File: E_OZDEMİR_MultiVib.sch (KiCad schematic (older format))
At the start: 11 parts, among them U1 MJB41C, U2 MJB41C

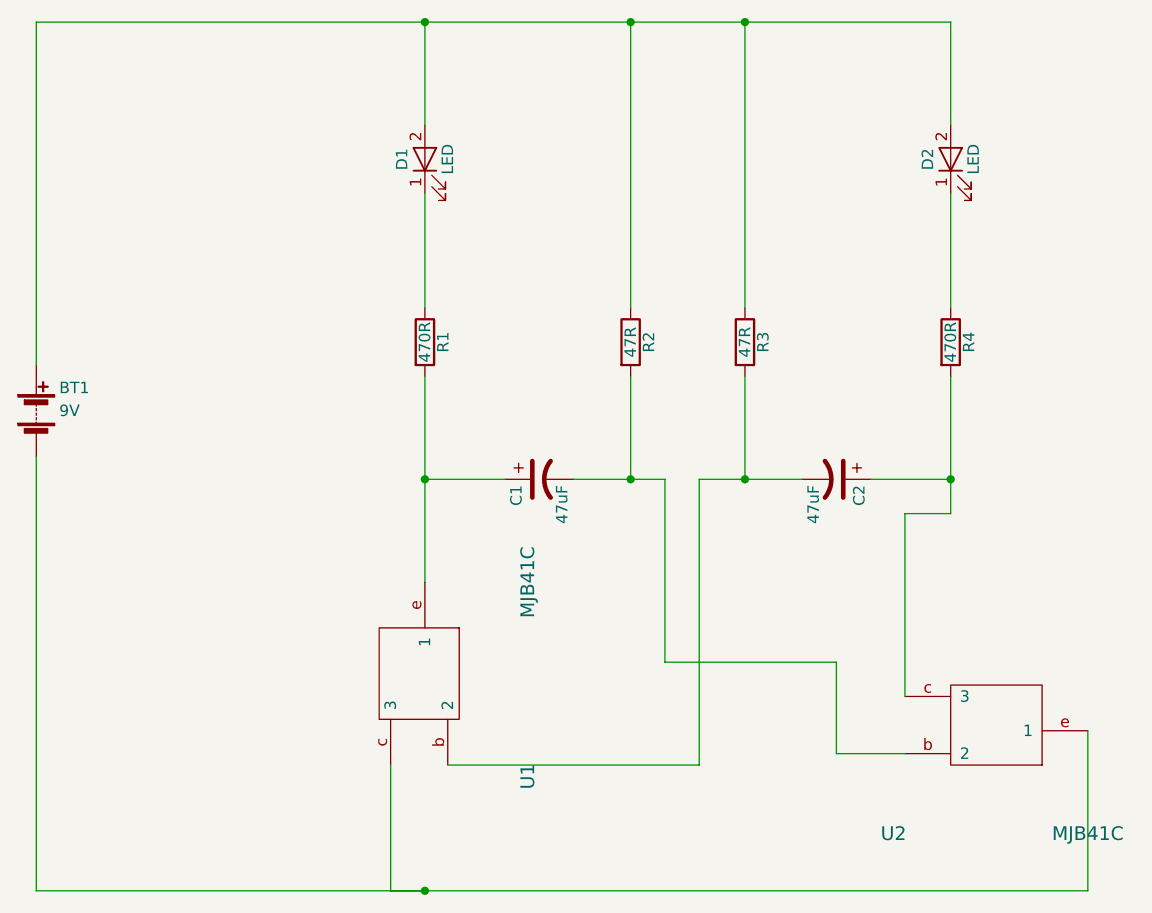
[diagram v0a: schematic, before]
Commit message: MultiVib
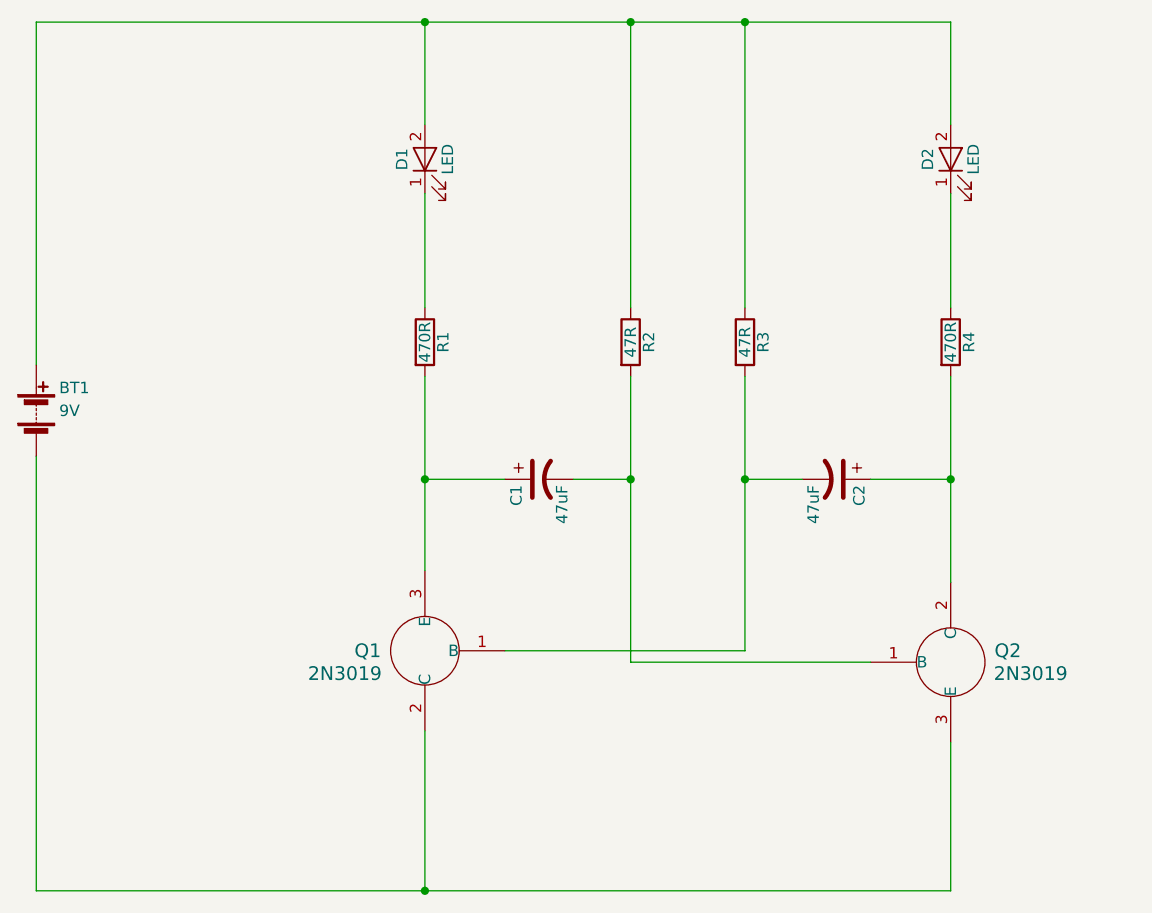
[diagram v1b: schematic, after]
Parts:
- removed U1, U2: MJB41C, symbol MJB41C
- added Q1, Q2: 2N3019, symbol 2N3019
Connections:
- net at C1.1, R1.2: now also Q1.3 (E)
- net at C1.2, R2.2: now also Q2.1 (B)
- net at C2.1, R4.2: now also Q2.2 (C)
- net at C2.2, R3.2: now also Q1.1 (B)
- net at BT1.2 (-): now also Q1.2 (C), Q2.3 (E)
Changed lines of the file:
@@
 LIBS:contrib
 LIBS:valves
-LIBS:MJB41C
+LIBS:2n3019
 LIBS:E_OZDEMİR_MultiVib-cache
 EELAYER 25 0
@@
 	3500 2900 3500 4800
 Wire Wire Line
-	3500 4800 8100 4800
-Connection ~ 5200 4800
-Wire Wire Line
-	6400 3000 6400 4250
-Wire Wire Line
-	6400 3000 6850 3000
-Wire Wire Line
-	5850 3000 6250 3000
-Wire Wire Line
-	6250 3000 6250 3800
-Wire Wire Line
-	6250 3800 7000 3800
-Wire Wire Line
-	7000 3800 7000 4200
-Wire Wire Line
-	6100 2550 6100 3000
-Connection ~ 6100 3000
-Wire Wire Line
-	6600 2550 6600 3000
-Connection ~ 6600 3000
-Wire Wire Line
 	3500 2500 3500 1000
 Wire Wire Line
@@
 	7150 3000 7500 3000
 Connection ~ 7500 3000
+Wire Wire Line
+	5200 2550 5200 3400
 $Comp
-L MJB41C U1
-U 1 1 58D84547
-P 5200 3850
-F 0 "U1" H 5650 4300 60  0000 C CNN
-F 1 "MJB41C" H 4800 4300 60  0000 C CNN
-F 2 "" H 5200 3850 60  0001 C CNN
-F 3 "http://www.farnell.com/datasheets/1750581.pdf?_ga=1.84896729.1568379178.1489696753" H 5200 3850 60  0001 C CNN
-	1    5200 3850
-	0    1    1    0
+L 2N3019 Q1
+U 1 1 59298EC6
+P 5200 3750
+F 0 "Q1" H 5450 3750 60  0000 C CNN
+F 1 "2N3019" H 5550 3850 60  0000 C CNN
+F 2 "" H 5750 3950 60  0001 C CNN
+F 3 "http://www.st.com/content/ccc/resource/technical/document/datasheet/e7/4a/c8/fd/63/61/43/0f/CD00003089.pdf/files/CD00003089.pdf/jcr:content/translations/en.CD00003089.pdf" H 5750 3950 60  0001 C CNN
+	1    5200 3750
+	-1   0    0    1
+$EndComp
+$Comp
+L 2N3019 Q2
+U 1 1 592990BB
+P 7500 3800
+F 0 "Q2" H 7750 3850 60  0000 C CNN
+F 1 "2N3019" H 7850 3750 60  0000 C CNN
+F 2 "" H 8050 4000 60  0001 C CNN
+F 3 "http://www.st.com/content/ccc/resource/technical/document/datasheet/e7/4a/c8/fd/63/61/43/0f/CD00003089.pdf/files/CD00003089.pdf/jcr:content/translations/en.CD00003089.pdf" H 8050 4000 60  0001 C CNN
+	1    7500 3800
+	1    0    0    -1
 $EndComp
 Wire Wire Line
-	5200 2550 5200 3450
+	5200 4100 5200 4800
+Connection ~ 5200 4800
 Wire Wire Line
-	6400 4250 5300 4250
+	3500 4800 7500 4800
 Wire Wire Line
-	5050 4250 5050 4800
+	7500 4800 7500 4150
 Wire Wire Line
-	5050 4800 5200 4800
+	7500 2550 7500 3450
 Wire Wire Line
-	7500 2550 7500 3150
-$Comp
-L MJB41C U2
-U 1 1 58D846D8
-P 7700 4100
-F 0 "U2" H 8150 4550 60  0000 C CNN
-F 1 "MJB41C" H 7300 4550 60  0000 C CNN
-F 2 "" H 7700 4100 60  0001 C CNN
-F 3 "http://www.farnell.com/datasheets/1750581.pdf?_ga=1.84896729.1568379178.1489696753" H 7700 4100 60  0001 C CNN
-	1    7700 4100
-	-1   0    0    1
-$EndComp
+	6600 3750 5550 3750
 Wire Wire Line
-	8100 4800 8100 4100
+	6600 2550 6600 3750
 Wire Wire Line
-	7000 4200 7300 4200
+	6600 3000 6850 3000
+Connection ~ 6600 3000
 Wire Wire Line
-	7300 3950 7300 3150
+	6100 3800 7150 3800
 Wire Wire Line
-	7300 3150 7500 3150
+	6100 2550 6100 3800
+Wire Wire Line
+	6100 3000 5850 3000
+Connection ~ 6100 3000
 $EndSCHEMATC
